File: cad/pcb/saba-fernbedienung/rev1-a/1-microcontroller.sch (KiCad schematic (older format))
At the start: 11 parts, among them J201 Conn_ARM_JTAG_SWD_10, Q201 BC856, U201 DOIT-DEVKITV1-ESP32-WROOM-32

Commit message: Add: Steuerschaltung, Codec, Audio
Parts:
- removed R207: 100, Resistor_SMD:R_0603_1608Metric, symbol Device:R
- removed U201: DOIT-DEVKITV1-ESP32-WROOM-32, RF_Module:ESP32-WROOM-32, symbol microcontroller:DOIT-DEVKITV1-ESP32-WROOM-32
- added U201: DOIT-DEVKITV1-ESP32-WROOM-32, RF_Module:ESP32-WROOM-32, symbol local:DOIT-DEVKITV1-ESP32-WROOM-32
- J201, Q201, R201, R203, R204, R205, R206: Placement No Place -> NP
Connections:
- net labels added: SABA_Schnelllauf, SPI_CS_LCD, SPI_CS_SDCARD, SPI_CS_VS1053, SPI_DCS_VS1053
- net labels removed: LCD_CS, SABA_Suchlauf_schnell, SDCARD_CS, VS1053_XCS, VS1053_XDCS
- wire segments 60 -> 59
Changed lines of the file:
@@
 $Descr A4 11693 8268
 encoding utf-8
-Sheet 2 3
+Sheet 2 7
 Title "Fernbedienung SABA 6-3D"
-Date "2021-01-11"
+Date "2021-01-13"
 Rev "1-A"
 Comp "Martin Wagner DL2WAG"
@@
 Comment4 "Fernbedienung für SABA \"Automatic\" Radios"
 $EndDescr
-$Comp
-L microcontroller:DOIT-DEVKITV1-ESP32-WROOM-32 U201
-U 1 1 5FFCAB8A
-P 2700 2900
-F 0 "U201" H 2400 4300 50  0000 C CNN
-F 1 "DOIT-DEVKITV1-ESP32-WROOM-32" H 3450 4300 50  0000 C CNN
-F 2 "RF_Module:ESP32-WROOM-32" H 2900 650 50  0001 C CNN
-F 3 "https://www.espressif.com/sites/default/files/documentation/esp32-wroom-32_datasheet_en.pdf" H 2400 2950 50  0001 C CNN
-	1    2700 2900
-	1    0    0    -1
-$EndComp
 Text GLabel 1700 1900 0    50   BiDi ~ 0
 ~RESET
@@
 	3300 3000 5550 3000
 Text GLabel 5550 3700 2    50   Output ~ 0
-VS1053_XDCS
+SPI_DCS_VS1053
 Text GLabel 5550 2200 2    50   Output ~ 0
-VS1053_XCS
+SPI_CS_VS1053
 Text GLabel 5550 2100 2    50   Input ~ 0
 VS1053_DREQ
@@
 LCD_A0
 Text GLabel 5550 2600 2    50   Output ~ 0
-LCD_CS
+SPI_CS_LCD
 Text GLabel 5550 3200 2    50   Output ~ 0
-SDCARD_CS
+SPI_CS_SDCARD
 NoConn ~ 3300 1800
 NoConn ~ 3300 2000
@@
 U 1 1 5FFDB025
 P 6650 2800
-F 0 "R201" V 6353 2800 50  0000 C CNN
-F 1 "10k" V 6444 2800 50  0000 C CNN
+F 0 "R201" V 6450 2800 50  0000 C CNN
+F 1 "10k" V 6550 2800 50  0000 C CNN
 F 2 "Resistor_SMD:R_0603_1608Metric" V 6580 2800 50  0001 C CNN
 F 3 "~" H 6650 2800 50  0001 C CNN
-F 4 "No Place" V 6535 2800 50  0000 C CNN "Placement"
+F 4 "NP" V 6650 2800 50  0000 C CNN "Placement"
 	1    6650 2800
 	0    1    1    0
@@
 Wire Wire Line
 	6500 2800 3300 2800
-$Comp
-L Transistor_BJT:BC856 Q201
-U 1 1 5FFDE545
-P 7100 2800
-F 0 "Q201" H 7291 2709 50  0000 L CNN
-F 1 "BC856" H 7291 2800 50  0000 L CNN
-F 2 "Package_TO_SOT_SMD:SOT-23" H 7300 2725 50  0001 L CIN
-F 3 "https://www.onsemi.com/pub/Collateral/BC860-D.pdf" H 7100 2800 50  0001 L CNN
-F 4 "No Place" H 7291 2891 50  0000 L CNN "Placement"
-	1    7100 2800
-	1    0    0    1
-$EndComp
 Wire Wire Line
 	6900 2800 6800 2800
@@
 Text GLabel 5550 2400 2    50   Output ~ 0
 SABA_Suchlauf_R
-Text GLabel 5550 2500 2    50   Output ~ 0
-SABA_Suchlauf_schnell
 Text GLabel 5550 2300 2    50   Output ~ 0
 SABA_Suchlauf_L
@@
 Wire Wire Line
 	3300 2400 4850 2400
-Wire Wire Line
-	5550 2400 5550 2500
 Text GLabel 5550 2700 2    50   Output ~ 0
 SABA_Mute
@@
 F 2 "" H 5750 5200 50  0001 C CNN
 F 3 "http://infocenter.arm.com/help/topic/com.arm.doc.ddi0314h/DDI0314H_coresight_components_trm.pdf" V 5400 3950 50  0001 C CNN
-F 4 "No Place" H 5500 5850 50  0000 C CNN "Placement"
+F 4 "NP" H 5500 5850 50  0000 C CNN "Placement"
 	1    5750 5200
 	-1   0    0    -1
@@
 F 2 "Resistor_SMD:R_0603_1608Metric" V 3880 4450 50  0001 C CNN
 F 3 "~" H 3950 4450 50  0001 C CNN
-F 4 "No Place" V 3900 4900 50  0000 R CNN "Placement"
+F 4 "NP" V 3950 4500 50  0000 R CNN "Placement"
 	1    3950 4450
 	-1   0    0    1
@@
 F 2 "Resistor_SMD:R_0603_1608Metric" V 4180 4450 50  0001 C CNN
 F 3 "~" H 4250 4450 50  0001 C CNN
-F 4 "No Place" V 4200 4900 50  0000 R CNN "Placement"
+F 4 "NP" V 4250 4500 50  0000 R CNN "Placement"
 	1    4250 4450
 	-1   0    0    1
@@
 F 2 "Resistor_SMD:R_0603_1608Metric" V 4780 4450 50  0001 C CNN
 F 3 "~" H 4850 4450 50  0001 C CNN
-F 4 "No Place" V 4800 4900 50  0000 R CNN "Placement"
+F 4 "NP" V 4850 4500 50  0000 R CNN "Placement"
 	1    4850 4450
 	-1   0    0    1
@@
 F 2 "Resistor_SMD:R_0603_1608Metric" V 4480 4450 50  0001 C CNN
 F 3 "~" H 4550 4450 50  0001 C CNN
-F 4 "No Place" V 4500 4900 50  0000 R CNN "Placement"
+F 4 "NP" V 4550 4500 50  0000 R CNN "Placement"
 	1    4550 4450
 	-1   0    0    1
@@
 Wire Wire Line
 	4550 4300 4550 2500
-Connection ~ 4550 2500
-Wire Wire Line
-	4550 2500 5550 2500
 Wire Wire Line
 	4850 4300 4850 2400
@@
 	4850 2400 5550 2400
 $Comp
-L Device:R R207
-U 1 1 60054E7A
-P 2800 1750
-F 0 "R207" H 2750 1600 50  0000 R CNN
-F 1 "100" H 2730 1750 50  0000 R CNN
-F 2 "Resistor_SMD:R_0603_1608Metric" V 2730 1750 50  0001 C CNN
-F 3 "~" H 2800 1750 50  0001 C CNN
-F 4 "No Place" V 2750 2200 50  0000 R CNN "Placement"
-	1    2800 1750
-	-1   0    0    1
+L local:DOIT-DEVKITV1-ESP32-WROOM-32 U201
+U 1 1 6045D6AE
+P 2700 2900
+F 0 "U201" H 2300 4300 50  0000 C CNN
+F 1 "DOIT-DEVKITV1-ESP32-WROOM-32" H 3400 4300 50  0000 C CNN
+F 2 "RF_Module:ESP32-WROOM-32" H 2900 650 50  0001 C CNN
+F 3 "" H 2400 2950 50  0001 C CNN
+	1    2700 2900
+	1    0    0    -1
+$EndComp
+Text GLabel 5550 2500 2    50   Output ~ 0
+SABA_Schnelllauf
+Wire Wire Line
+	4550 2500 5550 2500
+Connection ~ 4550 2500
+$Comp
+L Transistor_BJT:BC856 Q201
+U 1 1 5FFDE545
+P 7100 2800
+F 0 "Q201" H 7291 2709 50  0000 L CNN
+F 1 "BC856" H 7291 2800 50  0000 L CNN
+F 2 "Package_TO_SOT_SMD:SOT-23" H 7300 2725 50  0001 L CIN
+F 3 "https://www.onsemi.com/pub/Collateral/BC860-D.pdf" H 7100 2800 50  0001 L CNN
+F 4 "NP" H 7291 2891 50  0000 L CNN "Placement"
+	1    7100 2800
+	1    0    0    1
 $EndComp
 $EndSCHEMATC

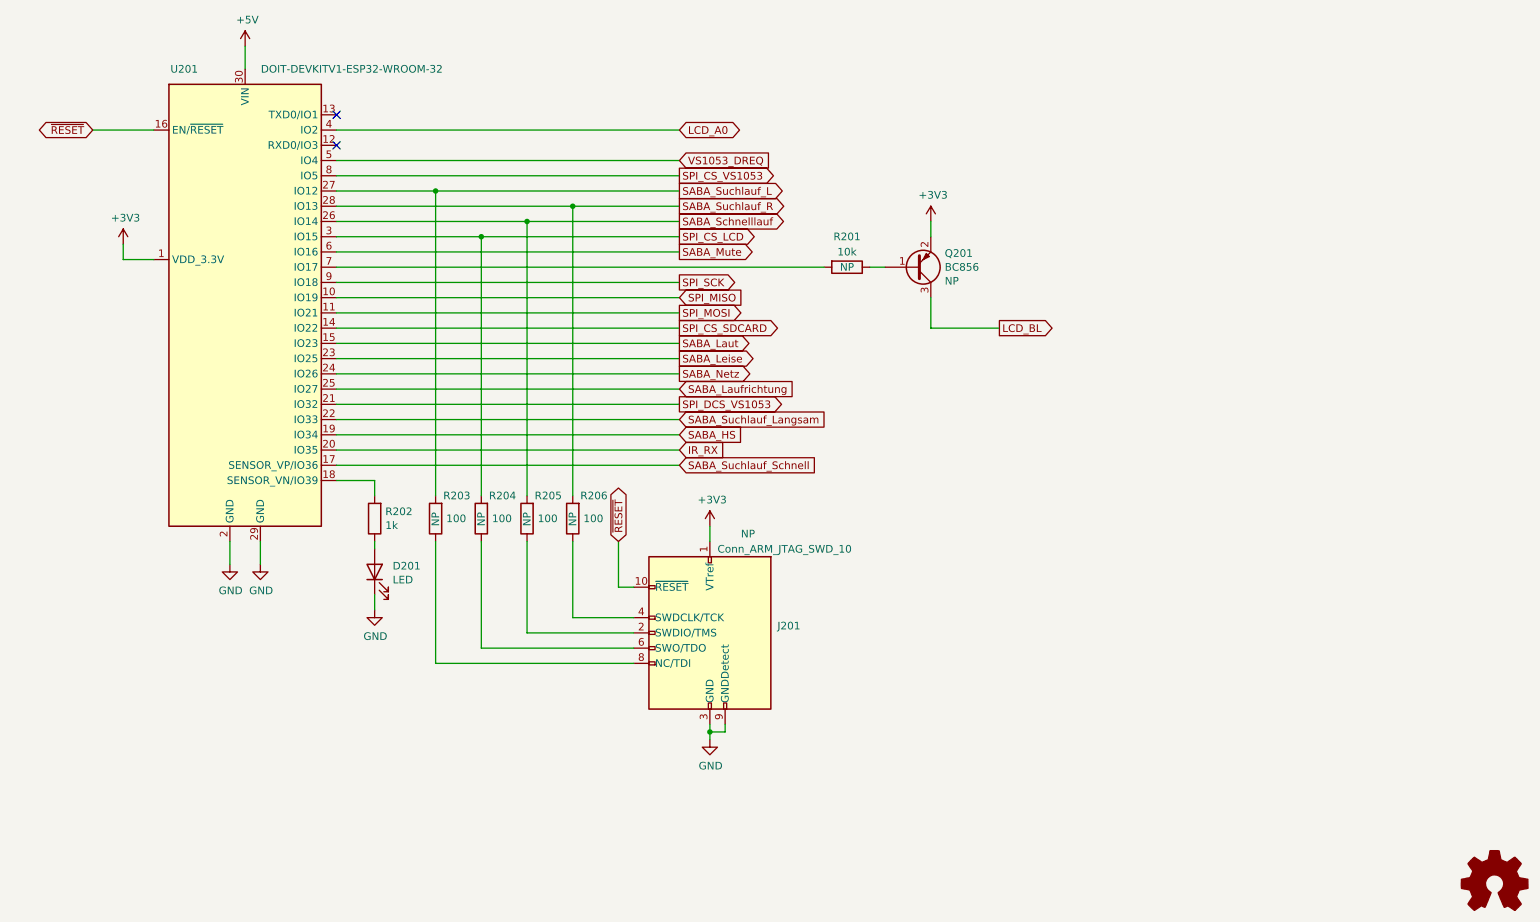
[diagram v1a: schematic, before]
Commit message: Fix: Div. DRC
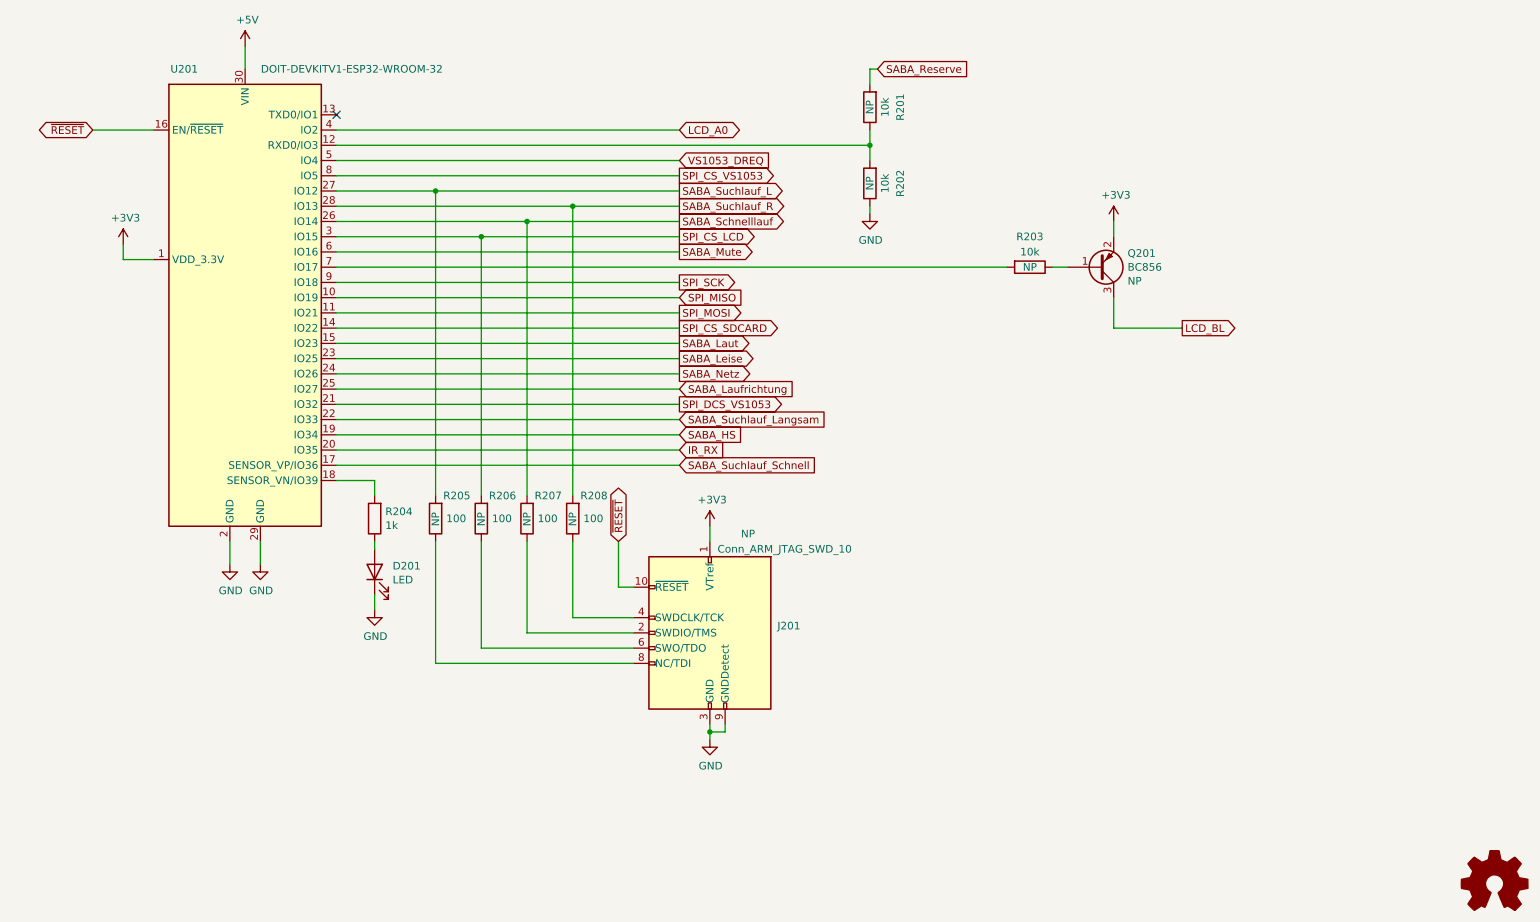
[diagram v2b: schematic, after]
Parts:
- added R201, R202: 10k, Resistor_SMD:R_0603_1608Metric, symbol Device:R
- renumbered R201 to R203, R202 to R204, R203 to R205, R204 to R206, R205 to R207, R206 to R208
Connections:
- net GND: now also R202.1
- net at U201.12 (RXD0/IO3): now also R201.1, R202.2
- new net SABA_Reserve: R201.2
- no-connect marks 2 -> 1
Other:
- moved on the sheet: Q201, R203
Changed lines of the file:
@@
 	1700 1900 2100 1900
 $Comp
-L power:GND #PWR0205
+L power:GND #PWR0206
 U 1 1 5FFCD50A
 P 2600 4750
-F 0 "#PWR0205" H 2600 4500 50  0001 C CNN
+F 0 "#PWR0206" H 2600 4500 50  0001 C CNN
 F 1 "GND" H 2605 4577 50  0000 C CNN
 F 2 "" H 2600 4750 50  0001 C CNN
@@
 $EndComp
 $Comp
-L power:GND #PWR0206
+L power:GND #PWR0207
 U 1 1 5FFCDB31
 P 2800 4750
-F 0 "#PWR0206" H 2800 4500 50  0001 C CNN
+F 0 "#PWR0207" H 2800 4500 50  0001 C CNN
 F 1 "GND" H 2805 4577 50  0000 C CNN
 F 2 "" H 2800 4750 50  0001 C CNN
@@
 	2800 4600 2800 4750
 $Comp
-L power:+3V3 #PWR0203
+L power:+3V3 #PWR0204
 U 1 1 5FFCE66A
 P 1900 2650
-F 0 "#PWR0203" H 1900 2500 50  0001 C CNN
+F 0 "#PWR0204" H 1900 2500 50  0001 C CNN
 F 1 "+3V3" H 1915 2823 50  0000 C CNN
 F 2 "" H 1900 2650 50  0001 C CNN
@@
 SPI_CS_SDCARD
 NoConn ~ 3300 1800
-NoConn ~ 3300 2000
 Wire Wire Line
 	5550 1900 3300 1900
@@
 	5550 4000 3300 4000
 $Comp
-L Device:R R201
+L Device:R R203
 U 1 1 5FFDB025
-P 6650 2800
-F 0 "R201" V 6450 2800 50  0000 C CNN
-F 1 "10k" V 6550 2800 50  0000 C CNN
-F 2 "Resistor_SMD:R_0603_1608Metric" V 6580 2800 50  0001 C CNN
-F 3 "~" H 6650 2800 50  0001 C CNN
-F 4 "NP" V 6650 2800 50  0000 C CNN "Placement"
-	1    6650 2800
+P 7850 2800
+F 0 "R203" V 7650 2800 50  0000 C CNN
+F 1 "10k" V 7750 2800 50  0000 C CNN
+F 2 "Resistor_SMD:R_0603_1608Metric" V 7780 2800 50  0001 C CNN
+F 3 "~" H 7850 2800 50  0001 C CNN
+F 4 "NP" V 7850 2800 50  0000 C CNN "Placement"
+	1    7850 2800
 	0    1    1    0
 $EndComp
 Wire Wire Line
-	6500 2800 3300 2800
-Wire Wire Line
-	6900 2800 6800 2800
-Wire Wire Line
-	7200 3000 7200 3200
-Wire Wire Line
-	7200 3200 7650 3200
-Text GLabel 7650 3200 2    50   Output ~ 0
+	7700 2800 3300 2800
+Wire Wire Line
+	8100 2800 8000 2800
+Wire Wire Line
+	8400 3000 8400 3200
+Wire Wire Line
+	8400 3200 8850 3200
+Text GLabel 8850 3200 2    50   Output ~ 0
 LCD_BL
 $Comp
-L power:+3V3 #PWR0202
+L power:+3V3 #PWR0203
 U 1 1 5FFE05B3
-P 7200 2500
-F 0 "#PWR0202" H 7200 2350 50  0001 C CNN
-F 1 "+3V3" H 7215 2673 50  0000 C CNN
-F 2 "" H 7200 2500 50  0001 C CNN
-F 3 "" H 7200 2500 50  0001 C CNN
-	1    7200 2500
-	1    0    0    -1
-$EndComp
-Wire Wire Line
-	7200 2500 7200 2600
+P 8400 2500
+F 0 "#PWR0203" H 8400 2350 50  0001 C CNN
+F 1 "+3V3" H 8415 2673 50  0000 C CNN
+F 2 "" H 8400 2500 50  0001 C CNN
+F 3 "" H 8400 2500 50  0001 C CNN
+	1    8400 2500
+	1    0    0    -1
+$EndComp
+Wire Wire Line
+	8400 2500 8400 2600
 Text GLabel 5550 3900 2    50   Input ~ 0
 SABA_HS
@@
 SABA_Suchlauf_Schnell
 $Comp
-L Device:R R202
+L Device:R R204
 U 1 1 5FFF2B18
 P 3550 4450
-F 0 "R202" H 3480 4404 50  0000 R CNN
+F 0 "R204" H 3480 4404 50  0000 R CNN
 F 1 "1k" H 3480 4495 50  0000 R CNN
 F 2 "Resistor_SMD:R_0603_1608Metric" V 3480 4450 50  0001 C CNN
@@
 	3550 4200 3300 4200
 $Comp
-L power:GND #PWR0207
+L power:GND #PWR0208
 U 1 1 5FFF784B
 P 3550 5050
-F 0 "#PWR0207" H 3550 4800 50  0001 C CNN
+F 0 "#PWR0208" H 3550 4800 50  0001 C CNN
 F 1 "GND" H 3555 4877 50  0000 C CNN
 F 2 "" H 3550 5050 50  0001 C CNN
@@
 ~RESET
 $Comp
-L power:+3V3 #PWR0204
+L power:+3V3 #PWR0205
 U 1 1 6001024E
 P 5750 4500
-F 0 "#PWR0204" H 5750 4350 50  0001 C CNN
+F 0 "#PWR0205" H 5750 4350 50  0001 C CNN
 F 1 "+3V3" H 5765 4673 50  0000 C CNN
 F 2 "" H 5750 4500 50  0001 C CNN
@@
 $EndComp
 $Comp
-L power:GND #PWR0208
+L power:GND #PWR0209
 U 1 1 60010E9A
 P 5750 5900
-F 0 "#PWR0208" H 5750 5650 50  0001 C CNN
+F 0 "#PWR0209" H 5750 5650 50  0001 C CNN
 F 1 "GND" H 5755 5727 50  0000 C CNN
 F 2 "" H 5750 5900 50  0001 C CNN
@@
 $EndComp
 $Comp
-L Device:R R203
+L Device:R R205
 U 1 1 6001163D
 P 3950 4450
-F 0 "R203" H 3900 4300 50  0000 R CNN
+F 0 "R205" H 3900 4300 50  0000 R CNN
 F 1 "100" H 3880 4450 50  0000 R CNN
 F 2 "Resistor_SMD:R_0603_1608Metric" V 3880 4450 50  0001 C CNN
@@
 $EndComp
 $Comp
-L Device:R R204
+L Device:R R206
 U 1 1 6001220B
 P 4250 4450
-F 0 "R204" H 4200 4300 50  0000 R CNN
+F 0 "R206" H 4200 4300 50  0000 R CNN
 F 1 "100" H 4180 4450 50  0000 R CNN
 F 2 "Resistor_SMD:R_0603_1608Metric" V 4180 4450 50  0001 C CNN
@@
 $EndComp
 $Comp
-L Device:R R206
+L Device:R R208
 U 1 1 60012608
 P 4850 4450
-F 0 "R206" H 4800 4300 50  0000 R CNN
+F 0 "R208" H 4800 4300 50  0000 R CNN
 F 1 "100" H 4780 4450 50  0000 R CNN
 F 2 "Resistor_SMD:R_0603_1608Metric" V 4780 4450 50  0001 C CNN
@@
 $EndComp
 $Comp
-L Device:R R205
+L Device:R R207
 U 1 1 60012995
 P 4550 4450
-F 0 "R205" H 4500 4300 50  0000 R CNN
+F 0 "R207" H 4500 4300 50  0000 R CNN
 F 1 "100" H 4480 4450 50  0000 R CNN
 F 2 "Resistor_SMD:R_0603_1608Metric" V 4480 4450 50  0001 C CNN
@@
 L Transistor_BJT:BC856 Q201
 U 1 1 5FFDE545
-P 7100 2800
-F 0 "Q201" H 7291 2709 50  0000 L CNN
-F 1 "BC856" H 7291 2800 50  0000 L CNN
-F 2 "Package_TO_SOT_SMD:SOT-23" H 7300 2725 50  0001 L CIN
-F 3 "https://www.onsemi.com/pub/Collateral/BC860-D.pdf" H 7100 2800 50  0001 L CNN
-F 4 "NP" H 7291 2891 50  0000 L CNN "Placement"
-	1    7100 2800
+P 8300 2800
+F 0 "Q201" H 8491 2709 50  0000 L CNN
+F 1 "BC856" H 8491 2800 50  0000 L CNN
+F 2 "Package_TO_SOT_SMD:SOT-23" H 8500 2725 50  0001 L CIN
+F 3 "https://www.onsemi.com/pub/Collateral/BC860-D.pdf" H 8300 2800 50  0001 L CNN
+F 4 "NP" H 8491 2891 50  0000 L CNN "Placement"
+	1    8300 2800
 	1    0    0    1
 $EndComp
+$Comp
+L Device:R R201
+U 1 1 60A2E32A
+P 6800 1750
+F 0 "R201" V 6600 1750 50  0000 C CNN
+F 1 "10k" V 6700 1750 50  0000 C CNN
+F 2 "Resistor_SMD:R_0603_1608Metric" V 6730 1750 50  0001 C CNN
+F 3 "~" H 6800 1750 50  0001 C CNN
+F 4 "NP" V 6800 1750 50  0000 C CNN "Placement"
+	1    6800 1750
+	-1   0    0    1
+$EndComp
+$Comp
+L Device:R R202
+U 1 1 60A2EA0B
+P 6800 2250
+F 0 "R202" V 6600 2250 50  0000 C CNN
+F 1 "10k" V 6700 2250 50  0000 C CNN
+F 2 "Resistor_SMD:R_0603_1608Metric" V 6730 2250 50  0001 C CNN
+F 3 "~" H 6800 2250 50  0001 C CNN
+F 4 "NP" V 6800 2250 50  0000 C CNN "Placement"
+	1    6800 2250
+	-1   0    0    1
+$EndComp
+Wire Wire Line
+	3300 2000 6800 2000
+Wire Wire Line
+	6800 1900 6800 2000
+Connection ~ 6800 2000
+Wire Wire Line
+	6800 2000 6800 2100
+Wire Wire Line
+	6800 2400 6800 2450
+Text GLabel 6850 1500 2    50   Input ~ 0
+SABA_Reserve
+Wire Wire Line
+	6800 1600 6800 1500
+$Comp
+L power:GND #PWR0202
+U 1 1 60A7B96C
+P 6800 2450
+F 0 "#PWR0202" H 6800 2200 50  0001 C CNN
+F 1 "GND" H 6805 2277 50  0000 C CNN
+F 2 "" H 6800 2450 50  0001 C CNN
+F 3 "" H 6800 2450 50  0001 C CNN
+	1    6800 2450
+	1    0    0    -1
+$EndComp
+Wire Wire Line
+	6800 1500 6850 1500
 $EndSCHEMATC

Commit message: New: Bauteil - Pad Zuordnungen
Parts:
- J201: footprint (none) -> Connector_PinHeader_1.27mm:PinHeader_2x05_P1.27mm_Vertical
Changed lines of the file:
@@
 F 0 "J201" H 5307 5246 50  0000 R CNN
 F 1 "Conn_ARM_JTAG_SWD_10" H 5700 5750 50  0000 R CNN
-F 2 "" H 5750 5200 50  0001 C CNN
+F 2 "Connector_PinHeader_1.27mm:PinHeader_2x05_P1.27mm_Vertical" H 5750 5200 50  0001 C CNN
 F 3 "http://infocenter.arm.com/help/topic/com.arm.doc.ddi0314h/DDI0314H_coresight_components_trm.pdf" V 5400 3950 50  0001 C CNN
 F 4 "NP" H 5500 5850 50  0000 C CNN "Placement"

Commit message: Fix: uC Gehaeuse
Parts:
- U201: footprint RF_Module:ESP32-WROOM-32 -> local:DOIT-DEVKITV1-ESP32-WROOM-32
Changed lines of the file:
@@
 F 0 "U201" H 2300 4300 50  0000 C CNN
 F 1 "DOIT-DEVKITV1-ESP32-WROOM-32" H 3400 4300 50  0000 C CNN
-F 2 "RF_Module:ESP32-WROOM-32" H 2900 650 50  0001 C CNN
+F 2 "local:DOIT-DEVKITV1-ESP32-WROOM-32" H 2900 650 50  0001 C CNN
 F 3 "" H 2400 2950 50  0001 C CNN
 	1    2700 2900

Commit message: Add: Bauteiltypen Digikey...
viele Bauteile von WE da hoffentlich lange gueltig...
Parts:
- D201: Bauteil (none) -> WE 150080BS75000
- Q201: Bauteil (none) -> ON BC856BLT1G
- U201: Bauteil (none) -> Doit ESP32 DEVKITV1 (Board mit ESP WROOM-32)
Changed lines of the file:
@@
 F 2 "LED_SMD:LED_0805_2012Metric" H 3550 4800 50  0001 C CNN
 F 3 "~" H 3550 4800 50  0001 C CNN
+F 4 "WE 150080BS75000" V 3550 4800 50  0001 C CNN "Bauteil"
 	1    3550 4800
 	0    -1   -1   0
@@
 F 2 "local:DOIT-DEVKITV1-ESP32-WROOM-32" H 2900 650 50  0001 C CNN
 F 3 "" H 2400 2950 50  0001 C CNN
+F 4 "Doit ESP32 DEVKITV1 (Board mit ESP WROOM-32)" H 2700 2900 50  0001 C CNN "Bauteil"
 	1    2700 2900
 	1    0    0    -1
@@
 F 1 "BC856" H 8491 2800 50  0000 L CNN
 F 2 "Package_TO_SOT_SMD:SOT-23" H 8500 2725 50  0001 L CIN
-F 3 "https://www.onsemi.com/pub/Collateral/BC860-D.pdf" H 8300 2800 50  0001 L CNN
+F 3 "" H 8300 2800 50  0001 L CNN
 F 4 "NP" H 8491 2891 50  0000 L CNN "Placement"
+F 5 "ON BC856BLT1G" H 8300 2800 50  0001 C CNN "Bauteil"
 	1    8300 2800
 	1    0    0    1
